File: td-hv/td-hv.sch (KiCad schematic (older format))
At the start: 43 parts, among them J1 Conn_01x07_Male, Q1 IMBF170R450M1XTMA1, U1 UCC2801, U2 TLC272, U3 LM2903

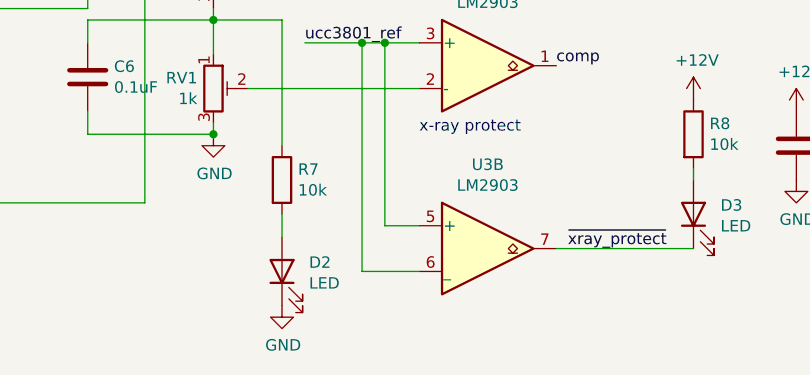
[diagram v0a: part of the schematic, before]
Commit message: pn updates for hv
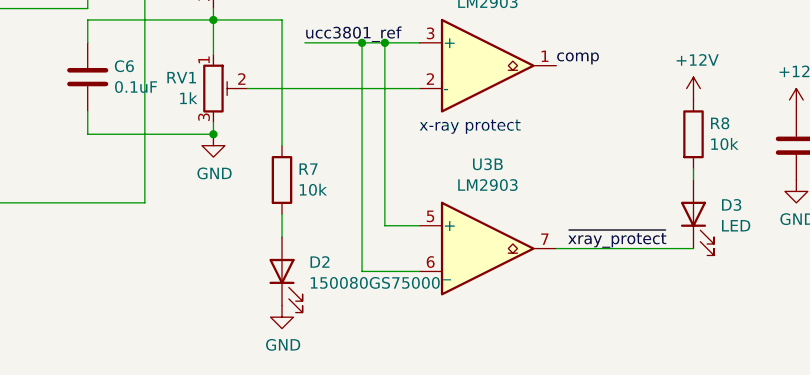
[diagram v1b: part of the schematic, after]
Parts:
- D2: value LED -> ‎150080GS75000‎; Digikey 732-4986-1-ND -> ‎732-4983-1-ND‎; Manufacturer (none) -> Würth Elektronik
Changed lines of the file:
@@
 P 8350 5650
 F 0 "D2" V 8389 5532 50  0000 R CNN
-F 1 "LED" V 8298 5532 50  0000 R CNN
+F 1 "‎150080GS75000‎" V 8298 5532 50  0000 R CNN
 F 2 "LED_SMD:LED_0805_2012Metric_Castellated" H 8350 5650 50  0001 C CNN
 F 3 "~" H 8350 5650 50  0001 C CNN
-F 4 "732-4986-1-ND" V 8350 5650 50  0001 C CNN "Digikey"
+F 4 " ‎732-4983-1-ND‎ " V 8350 5650 50  0001 C CNN "Digikey"
+F 5 " Würth Elektronik" V 8350 5650 50  0001 C CNN "Manufacturer"
 	1    8350 5650
 	0    -1   -1   0
